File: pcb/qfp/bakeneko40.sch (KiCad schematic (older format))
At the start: 116 parts, among them J1 JST SH 4-pin, J2 AVR-ISP-6, SW1 SW_Push, U1 ATmega32U2-AU, U2 SRV05-4, Y1 16MHz

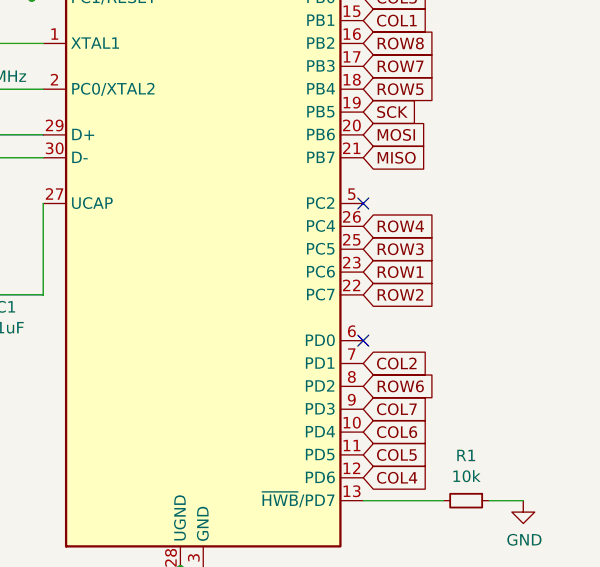
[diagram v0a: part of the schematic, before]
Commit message: pcb and qmk edits
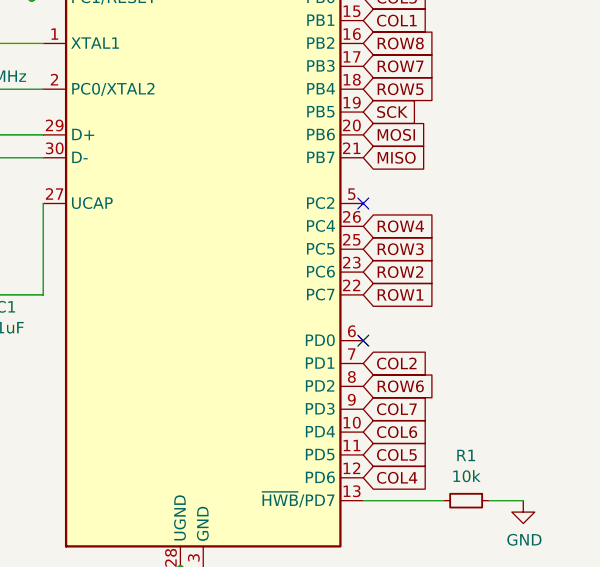
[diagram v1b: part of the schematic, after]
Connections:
- net ROW1: now also U1.22 (PC7); no longer U1.23 (PC6)
- net ROW2: now also U1.23 (PC6); no longer U1.22 (PC7)
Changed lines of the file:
@@
 Wire Wire Line
 	8750 1900 8750 2050
-Text GLabel 10200 3250 2    50   Input ~ 0
-ROW1
 Text GLabel 10200 2650 2    50   Input ~ 0
 MOSI
 Text GLabel 10200 3750 2    50   Input ~ 0
 ROW6
-Text GLabel 10200 3350 2    50   Input ~ 0
-ROW2
 Wire Wire Line
 	9050 4550 9400 4550
@@
 NoConn ~ 10200 3550
 NoConn ~ 10200 2950
+Text GLabel 10200 3350 2    50   Input ~ 0
+ROW1
+Text GLabel 10200 3250 2    50   Input ~ 0
+ROW2
 $EndSCHEMATC
